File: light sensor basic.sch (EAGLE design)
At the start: 1 part

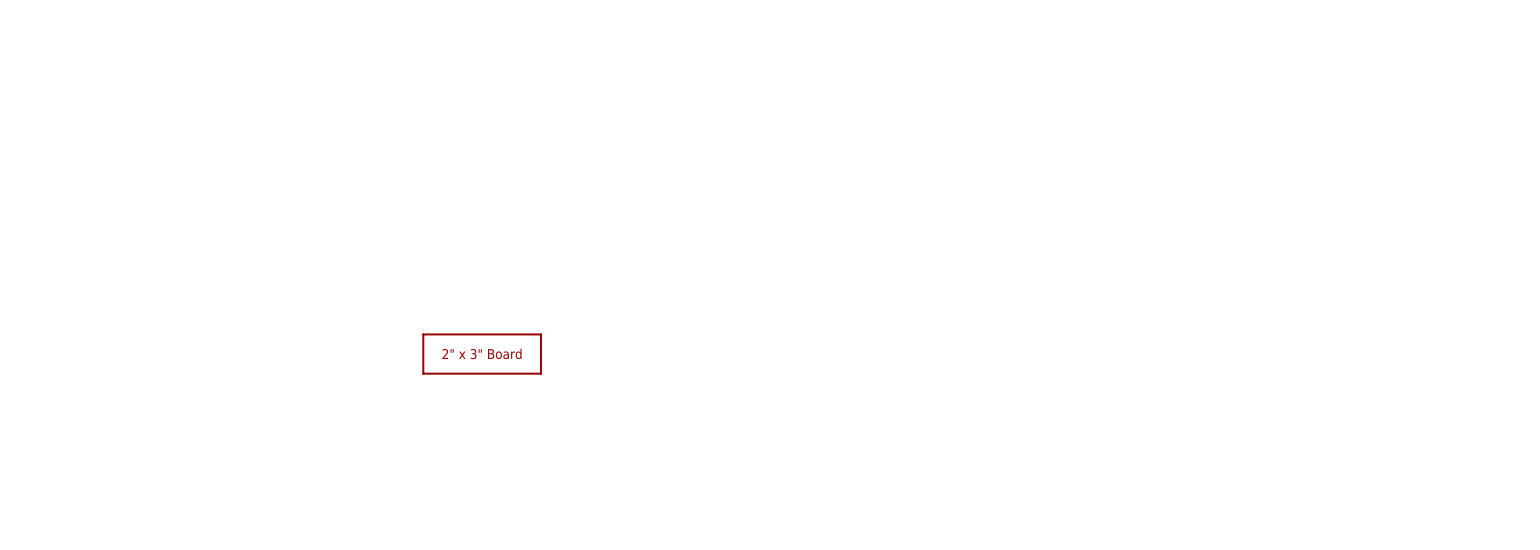
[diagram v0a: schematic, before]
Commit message: Eagle 2
Eagle 2
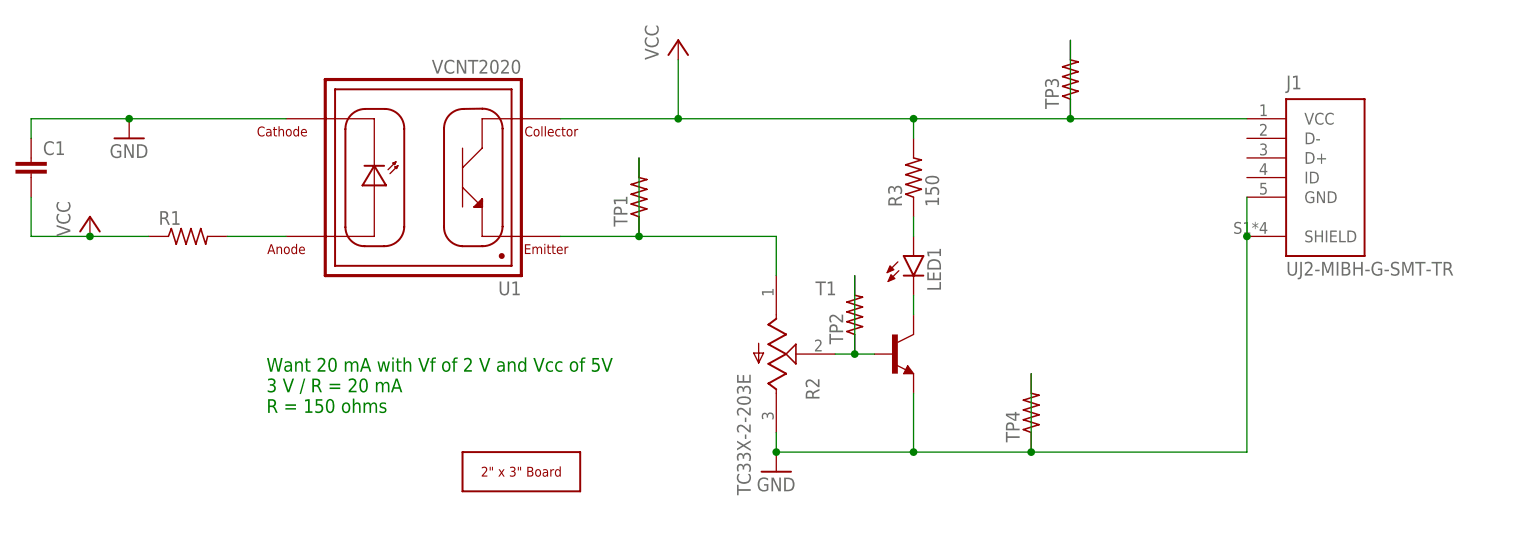
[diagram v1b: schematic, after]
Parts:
- added C1: (no value), rcl:C-EUC1206
- added J1: UJ2-MIBH-G-SMT-TR, UJ2-MIBH-G-SMT-TR:UJ2-MIBH-G-SMT-TR
- added LED1: (no value), led:LEDSML0805
- added R1, TP1, TP2, TP3, TP4: (no value), rcl:R-US_R1206
- added R2: TC33X-2-203E, TC33X-2-203E:TC33X-2-203E
- added R3: 150, rcl:R-US_R0805
- added T1: (no value), transistor:-NPN-SOT23-EBC
- added U1: VCNT2020, VCNT2020:VCNT2020
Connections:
- new net GND: C1.1, J1.GND, J1.SHIELD, R2.CW, T1.E, TP4.1, TP4.2, U1.CATHODE
- new net N$1: R1.2, U1.ANODE
- new net N$3: R2.W, T1.B, TP2.1, TP2.2
- new net N$4: LED1.A, R3.1
- new net N$5: LED1.C, T1.C
- new net TP1: R2.CCW, TP1.1, TP1.2, U1.EMITTER
- new net VCC: C1.2, J1.VCC, R1.1, R3.2, TP3.1, TP3.2, U1.COLLECTOR
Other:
- note added: "Want 20 mA with Vf of 2 V and Vcc of 5V 3 V / R = 20 mA R = 150 ohms"
